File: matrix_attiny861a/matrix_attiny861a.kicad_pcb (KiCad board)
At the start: 2 copper layers, 16 x 29 mm, 9 parts, among them IC1 ATTINY861A-S

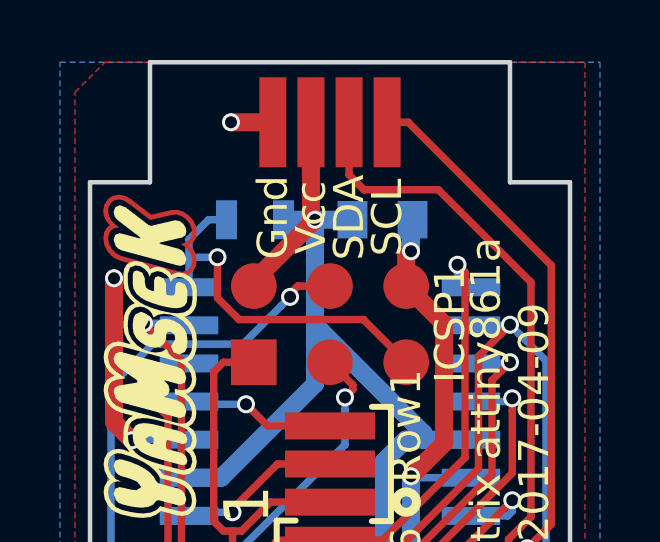
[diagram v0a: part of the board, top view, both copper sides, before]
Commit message: bugfixes preparing first order to oshpark
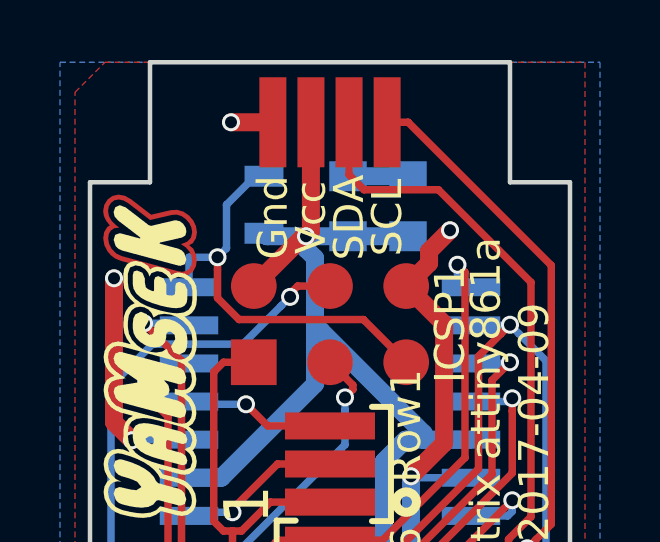
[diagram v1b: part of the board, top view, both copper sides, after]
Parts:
- added C2: 0.1µF, Capacitors_SMD:C_0805, B.Cu at (50.6, 49.8)
- moved C1 0.96 mm to (52.6, 49.8), turned to 90 degrees
- moved R1 0.58 mm to (47.8, 49.8), turned to 270 degrees
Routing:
- net GND: track 34.6 -> 36.8 mm
- net +5V: track 43.9 -> 46.0 mm
- net /Rst: track 12.6 -> 14.0 mm
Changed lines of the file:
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@@
 (kicad_pcb (version 4) (host pcbnew 4.0.5+dfsg1-4)
   (general
-    (links 37)
+    (links 39)
     (no_connects 0)
     (area 41.924999 44.924999 58.075001 74.075001)
     (thickness 1.6)
     (drawings 28)
-    (tracks 284)
+    (tracks 289)
     (zones 0)
-    (modules 9)
+    (modules 10)
     (nets 19)
   )
@@
     (46 B.CrtYd user hide)
     (47 F.CrtYd user)
-    (48 B.Fab user hide)
-    (49 F.Fab user hide)
+    (48 B.Fab user)
+    (49 F.Fab user)
   )
   (setup
-    (last_trace_width 0.25)
+    (last_trace_width 0.6)
     (user_trace_width 0.6)
     (trace_clearance 0.2)
@@
   )
   (module Resistors_SMD:R_0805 (layer B.Cu)
-    (at 47.5 50.25)
+    (at 47.8 49.75 270)
     (descr "Resistor SMD 0805, reflow soldering, Vishay (see dcrcw.pdf)")
     (tags "resistor 0805")
     (attr smd)
-    (fp_text reference R1 (at 2.254999 0.065) (layer B.Fab)
+    (fp_text reference R1 (at -2.15 0 270) (layer B.Fab)
       (effects (font (size 1 1) (thickness 0.15)) (justify mirror))
     )
-    (fp_text value 10K (at 0.004999 0.065 90) (layer B.SilkS)
+    (fp_text value 10K (at 0.004999 0.065 360) (layer B.SilkS)
       (effects (font (size 0.5 0.5) (thickness 0.125)) (justify mirror))
     )
@@
     (fp_line (start 0.6 -0.875) (end -0.6 -0.875) (layer B.SilkS) (width 0.15))
     (fp_line (start -0.6 0.875) (end 0.6 0.875) (layer B.SilkS) (width 0.15))
-    (pad 1 smd rect (at -0.95 0) (size 0.7 1.3) (layers B.Cu B.Paste B.Mask)
+    (pad 1 smd rect (at -0.95 0 270) (size 0.7 1.3) (layers B.Cu B.Paste B.Mask)
       (net 11 /Rst))
-    (pad 2 smd rect (at 0.95 0) (size 0.7 1.3) (layers B.Cu B.Paste B.Mask)
+    (pad 2 smd rect (at 0.95 0 270) (size 0.7 1.3) (layers B.Cu B.Paste B.Mask)
       (net 8 +5V))
     (model Resistors_SMD.3dshapes/R_0805.wrl
@@
   )
   (module Capacitors_SMD:C_0805 (layer B.Cu)
-    (at 51.75 50.25)
+    (at 52.6 49.8 90)
     (descr "Capacitor SMD 0805, reflow soldering, AVX (see smccp.pdf)")
     (tags "capacitor 0805")
     (attr smd)
-    (fp_text reference C1 (at 0 2.1) (layer B.SilkS)
+    (fp_text reference C1 (at 2.25 -0.05 90) (layer B.Fab)
       (effects (font (size 1 1) (thickness 0.15)) (justify mirror))
     )
-    (fp_text value 10µF (at 0 -2.1) (layer B.Fab)
-      (effects (font (size 1 1) (thickness 0.15)) (justify mirror))
+    (fp_text value 10µF (at 0 -0.05 360) (layer B.SilkS)
+      (effects (font (size 0.5 0.5) (thickness 0.125)) (justify mirror))
     )
     (fp_line (start -1 -0.625) (end -1 0.625) (layer B.Fab) (width 0.15))
@@
     (fp_line (start 0.5 0.85) (end -0.5 0.85) (layer B.SilkS) (width 0.15))
     (fp_line (start -0.5 -0.85) (end 0.5 -0.85) (layer B.SilkS) (width 0.15))
-    (pad 1 smd rect (at -1 0) (size 1 1.25) (layers B.Cu B.Paste B.Mask)
+    (pad 1 smd rect (at -1 0 90) (size 1 1.25) (layers B.Cu B.Paste B.Mask)
       (net 8 +5V))
-    (pad 2 smd rect (at 1 0) (size 1 1.25) (layers B.Cu B.Paste B.Mask)
+    (pad 2 smd rect (at 1 0 90) (size 1 1.25) (layers B.Cu B.Paste B.Mask)
       (net 12 GND))
     (model Capacitors_SMD.3dshapes/C_0805.wrl
@@
       (xy 4.845618 -1.561278) (xy 4.849469 -1.565096)) (layer F.Cu) (width 0))
   )
+  (module Capacitors_SMD:C_0805 (layer B.Cu)
+    (at 50.6 49.8 90)
+    (descr "Capacitor SMD 0805, reflow soldering, AVX (see smccp.pdf)")
+    (tags "capacitor 0805")
+    (attr smd)
+    (fp_text reference C2 (at 2.4 0 90) (layer B.Fab)
+      (effects (font (size 1 1) (thickness 0.15)) (justify mirror))
+    )
+    (fp_text value 0.1µF (at 0 0.2 360) (layer B.SilkS)
+      (effects (font (size 0.5 0.5) (thickness 0.125)) (justify mirror))
+    )
+    (fp_line (start -1 -0.625) (end -1 0.625) (layer B.Fab) (width 0.15))
+    (fp_line (start 1 -0.625) (end -1 -0.625) (layer B.Fab) (width 0.15))
+    (fp_line (start 1 0.625) (end 1 -0.625) (layer B.Fab) (width 0.15))
+    (fp_line (start -1 0.625) (end 1 0.625) (layer B.Fab) (width 0.15))
+    (fp_line (start -1.8 1) (end 1.8 1) (layer B.CrtYd) (width 0.05))
+    (fp_line (start -1.8 -1) (end 1.8 -1) (layer B.CrtYd) (width 0.05))
+    (fp_line (start -1.8 1) (end -1.8 -1) (layer B.CrtYd) (width 0.05))
+    (fp_line (start 1.8 1) (end 1.8 -1) (layer B.CrtYd) (width 0.05))
+    (fp_line (start 0.5 0.85) (end -0.5 0.85) (layer B.SilkS) (width 0.15))
+    (fp_line (start -0.5 -0.85) (end 0.5 -0.85) (layer B.SilkS) (width 0.15))
+    (pad 1 smd rect (at -1 0 90) (size 1 1.25) (layers B.Cu B.Paste B.Mask)
+      (net 8 +5V))
+    (pad 2 smd rect (at 1 0 90) (size 1 1.25) (layers B.Cu B.Paste B.Mask)
+      (net 12 GND))
+    (model Capacitors_SMD.3dshapes/C_0805.wrl
+      (at (xyz 0 0 0))
+      (scale (xyz 1 1 1))
+      (rotate (xyz 0 0 0))
+    )
+  )
   (gr_text "matrix attiny861a\n2017-04-09" (at 56 57 90) (layer F.SilkS)
     (effects (font (size 1 1) (thickness 0.2)))
@@
   (segment (start 46.124999 55.323001) (end 46.448 55) (width 0.25) (layer F.Cu) (net 7))
   (segment (start 46.448 55) (end 47.46 55) (width 0.25) (layer F.Cu) (net 7))
+  (segment (start 49.200006 50.8) (end 47.9 50.8) (width 0.6) (layer B.Cu) (net 8))
+  (segment (start 47.9 50.8) (end 47.8 50.7) (width 0.6) (layer B.Cu) (net 8))
+  (segment (start 52.6 50.8) (end 50.6 50.8) (width 0.6) (layer B.Cu) (net 8))
+  (segment (start 50.6 50.8) (end 49.200006 50.8) (width 0.6) (layer B.Cu) (net 8))
+  (segment (start 49.365 50.635006) (end 49.200006 50.8) (width 0.6) (layer F.Cu) (net 8))
+  (segment (start 49.12 50.8) (end 49.200006 50.8) (width 0.6) (layer F.Cu) (net 8))
+  (segment (start 49.365 47) (end 49.365 50.635006) (width 0.6) (layer F.Cu) (net 8))
+  (segment (start 49.200006 51.224264) (end 49.200006 50.8) (width 0.6) (layer B.Cu) (net 8))
+  (segment (start 49.5 51.524258) (end 49.200006 51.224264) (width 0.6) (layer B.Cu) (net 8))
+  (segment (start 47.46 52.46) (end 49.12 50.8) (width 0.6) (layer F.Cu) (net 8))
+  (segment (start 49.5 53.955) (end 49.5 51.524258) (width 0.6) (layer B.Cu) (net 8))
+  (via (at 49.200006 50.8) (size 0.6) (drill 0.4) (layers F.Cu B.Cu) (net 8))
   (segment (start 53.125 57.58) (end 53.125 57.375) (width 0.6) (layer B.Cu) (net 8))
   (segment (start 53.125 57.375) (end 49.705 53.955) (width 0.6) (layer B.Cu) (net 8))
@@
   (segment (start 45.3 58.85) (end 46.378613 58.85) (width 0.6) (layer B.Cu) (net 8))
   (segment (start 54.7 57.58) (end 53.125 57.58) (width 0.6) (layer B.Cu) (net 8))
-  (segment (start 49.5 53.955) (end 49.5 50.25) (width 0.6) (layer B.Cu) (net 8))
-  (segment (start 47.46 52.46) (end 47.46 52.29) (width 0.6) (layer F.Cu) (net 8))
-  (segment (start 47.46 52.29) (end 49.5 50.25) (width 0.6) (layer F.Cu) (net 8))
-  (segment (start 49.5 50.25) (end 48.45 50.25) (width 0.6) (layer B.Cu) (net 8))
-  (segment (start 49.5 50.25) (end 50.75 50.25) (width 0.6) (layer B.Cu) (net 8))
-  (segment (start 49.365 47) (end 49.365 50.115) (width 0.6) (layer F.Cu) (net 8))
-  (segment (start 49.365 50.115) (end 49.5 50.25) (width 0.6) (layer F.Cu) (net 8))
-  (via (at 49.5 50.25) (size 0.6) (drill 0.4) (layers F.Cu B.Cu) (net 8))
   (segment (start 50.2 61.4) (end 50.19 61.39) (width 0.25) (layer B.Cu) (net 9))
   (segment (start 50.19 61.39) (end 46.86 61.39) (width 0.25) (layer B.Cu) (net 9))
@@
   (segment (start 48.36937 53.120697) (end 48.669369 52.820698) (width 0.25) (layer B.Cu) (net 10))
   (via (at 48.669369 52.820698) (size 0.6) (drill 0.4) (layers F.Cu B.Cu) (net 10))
+  (segment (start 46.25 51.5) (end 46.549999 51.200001) (width 0.25) (layer B.Cu) (net 11))
+  (segment (start 46.549999 51.200001) (end 46.549999 49.750001) (width 0.25) (layer B.Cu) (net 11))
+  (segment (start 46.549999 49.750001) (end 47.5 48.8) (width 0.25) (layer B.Cu) (net 11))
+  (segment (start 47.5 48.8) (end 47.8 48.8) (width 0.25) (layer B.Cu) (net 11))
   (segment (start 46.967973 53.576735) (end 46.25 52.858762) (width 0.25) (layer F.Cu) (net 11))
   (segment (start 46.25 52.858762) (end 46.25 51.924264) (width 0.25) (layer F.Cu) (net 11))
@@
   (segment (start 51.116735 53.576735) (end 46.967973 53.576735) (width 0.25) (layer F.Cu) (net 11))
   (segment (start 45.3 52.5) (end 45.3 51.5) (width 0.25) (layer B.Cu) (net 11))
-  (segment (start 45.3 51.5) (end 45.3 50.9) (width 0.25) (layer B.Cu) (net 11))
   (segment (start 46.25 51.5) (end 45.3 51.5) (width 0.25) (layer B.Cu) (net 11))
   (via (at 46.25 51.5) (size 0.6) (drill 0.4) (layers F.Cu B.Cu) (net 11))
-  (segment (start 45.3 50.9) (end 45.95 50.25) (width 0.25) (layer B.Cu) (net 11))
-  (segment (start 45.95 50.25) (end 46.55 50.25) (width 0.25) (layer B.Cu) (net 11))
+  (segment (start 53.301999 51.298001) (end 54 50.6) (width 0.6) (layer F.Cu) (net 12))
+  (segment (start 53.301999 51.698001) (end 53.301999 51.298001) (width 0.6) (layer F.Cu) (net 12))
+  (segment (start 52.54 52.46) (end 53.301999 51.698001) (width 0.6) (layer F.Cu) (net 12))
+  (via (at 54 50.6) (size 0.6) (drill 0.4) (layers F.Cu B.Cu) (net 12))
+  (segment (start 52.6 48.8) (end 50.6 48.8) (width 0.6) (layer B.Cu) (net 12))
   (segment (start 43.4 57.6) (end 42.8 57) (width 0.6) (layer F.Cu) (net 12))
   (segment (start 42.8 57) (end 42.8 52.2) (width 0.6) (layer F.Cu) (net 12))
@@
   (segment (start 55.707001 69.394239) (end 55.050761 68.737999) (width 0.6) (layer F.Cu) (net 12))
   (segment (start 54.9 68.737999) (end 54.9 66.5) (width 0.6) (layer F.Cu) (net 12))
-  (segment (start 52.7 51.3) (end 52.7 50.3) (width 0.6) (layer B.Cu) (net 12))
-  (segment (start 52.7 50.3) (end 52.75 50.25) (width 0.6) (layer B.Cu) (net 12))
-  (segment (start 52.54 52.46) (end 52.54 51.46) (width 0.6) (layer F.Cu) (net 12))
-  (segment (start 52.54 51.46) (end 52.7 51.3) (width 0.6) (layer F.Cu) (net 12))
-  (via (at 52.7 51.3) (size 0.6) (drill 0.4) (layers F.Cu B.Cu) (net 12))
   (segment (start 52.7 58.8) (end 52.7 64.3) (width 0.6) (layer B.Cu) (net 12))
   (segment (start 52.7 64.3) (end 54.9 66.5) (width 0.6) (layer B.Cu) (net 12))
